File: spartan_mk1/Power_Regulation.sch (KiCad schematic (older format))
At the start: 29 parts, among them J14 Conn_01x02_Female, Q3 AO3401A, U5 NCP1117-3.3_TO252, U6 TPS5430DDA

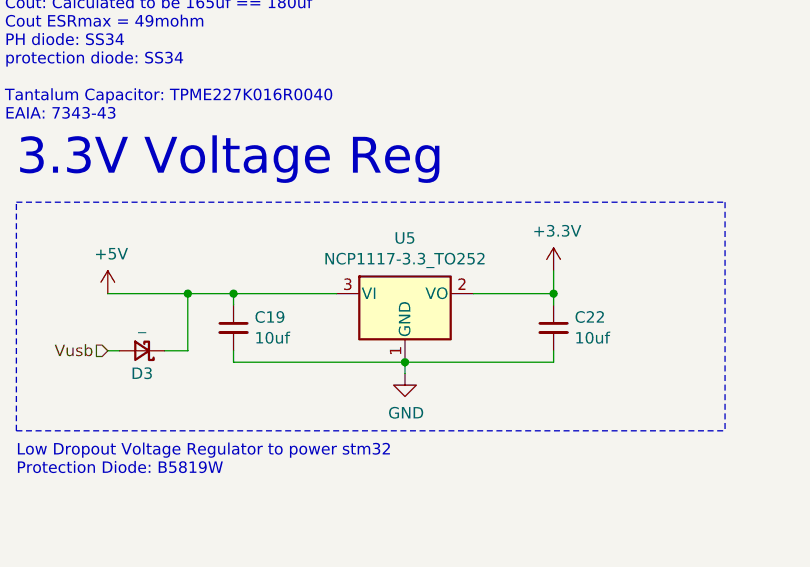
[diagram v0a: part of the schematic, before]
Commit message: updated placement
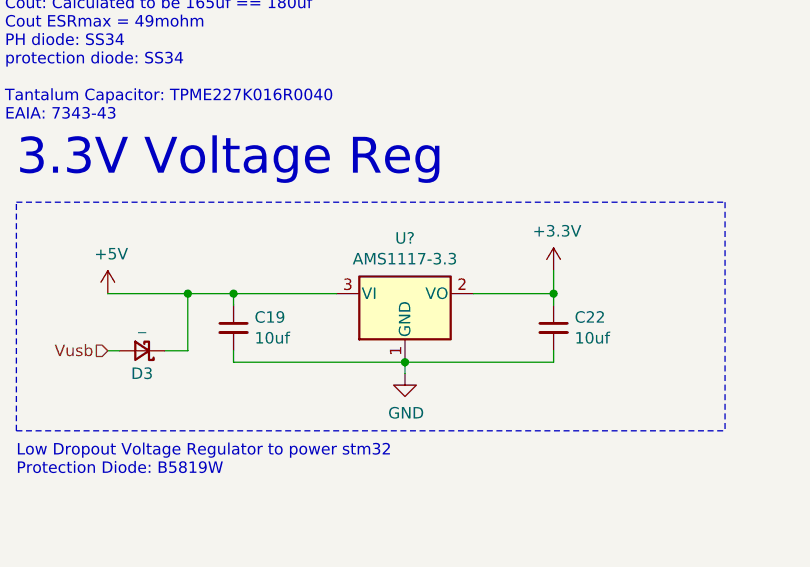
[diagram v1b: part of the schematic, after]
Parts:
- removed U5: NCP1117-3.3_TO252, Package_TO_SOT_SMD:TO-252-2, symbol Regulator_Linear:NCP1117-3.3_TO252
- added U?: AMS1117-3.3, Package_TO_SOT_SMD:SOT-223-3_TabPin2, symbol Regulator_Linear:AMS1117-3.3
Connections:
- net +3V3: now also U?.2 (VO)
- net +5V: now also U?.3 (VI)
- net GND: now also U?.1 (GND)
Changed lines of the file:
@@
 Low Dropout Voltage Regulator to power stm32\nProtection Diode: B5819W
-$Comp
-L Regulator_Linear:NCP1117-3.3_TO252 U?
-U 1 1 5F7A601F
-P 7850 4400
-AR Path="/5F78701C/5F7A601F" Ref="U?"  Part="1"
-AR Path="/5F79A745/5F7A601F" Ref="U5"  Part="1"
-F 0 "U5" H 7850 4642 50  0000 C CNN
-F 1 "NCP1117-3.3_TO252" H 7850 4551 50  0000 C CNN
-F 2 "Package_TO_SOT_SMD:TO-252-2" H 7850 4625 50  0001 C CNN
-F 3 "http://www.onsemi.com/pub_link/Collateral/NCP1117-D.PDF" H 7850 4400 50  0001 C CNN
-	1    7850 4400
-	1    0    0    -1
-$EndComp
 $Comp
 L Device:LED_Small D?
@@
 Wire Wire Line
 	7300 1350 7900 1350
+$Comp
+L Regulator_Linear:AMS1117-3.3 U?
+U 1 1 5FA17F2E
+P 7850 4400
+F 0 "U?" H 7850 4642 50  0000 C CNN
+F 1 "AMS1117-3.3" H 7850 4551 50  0000 C CNN
+F 2 "Package_TO_SOT_SMD:SOT-223-3_TabPin2" H 7850 4600 50  0001 C CNN
+F 3 "http://www.advanced-monolithic.com/pdf/ds1117.pdf" H 7950 4150 50  0001 C CNN
+	1    7850 4400
+	1    0    0    -1
+$EndComp
 $EndSCHEMATC
